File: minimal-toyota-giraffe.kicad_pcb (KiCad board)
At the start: 2 copper layers, 39.4 x 24.1 mm, 6 parts, among them J1 USB_A, J2 MOBILEEYE, J3 MOBILEEYE, P1 panda, U1 Power

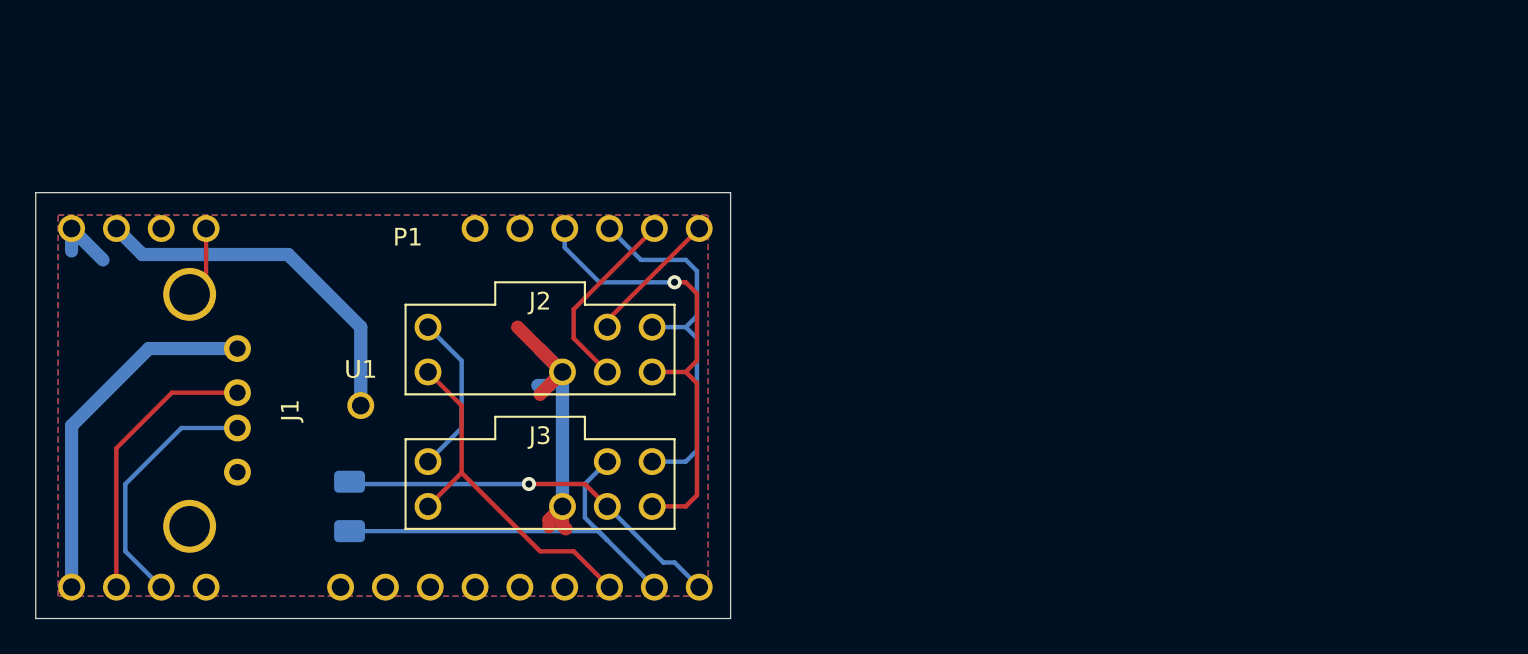
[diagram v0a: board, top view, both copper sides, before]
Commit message: new board design
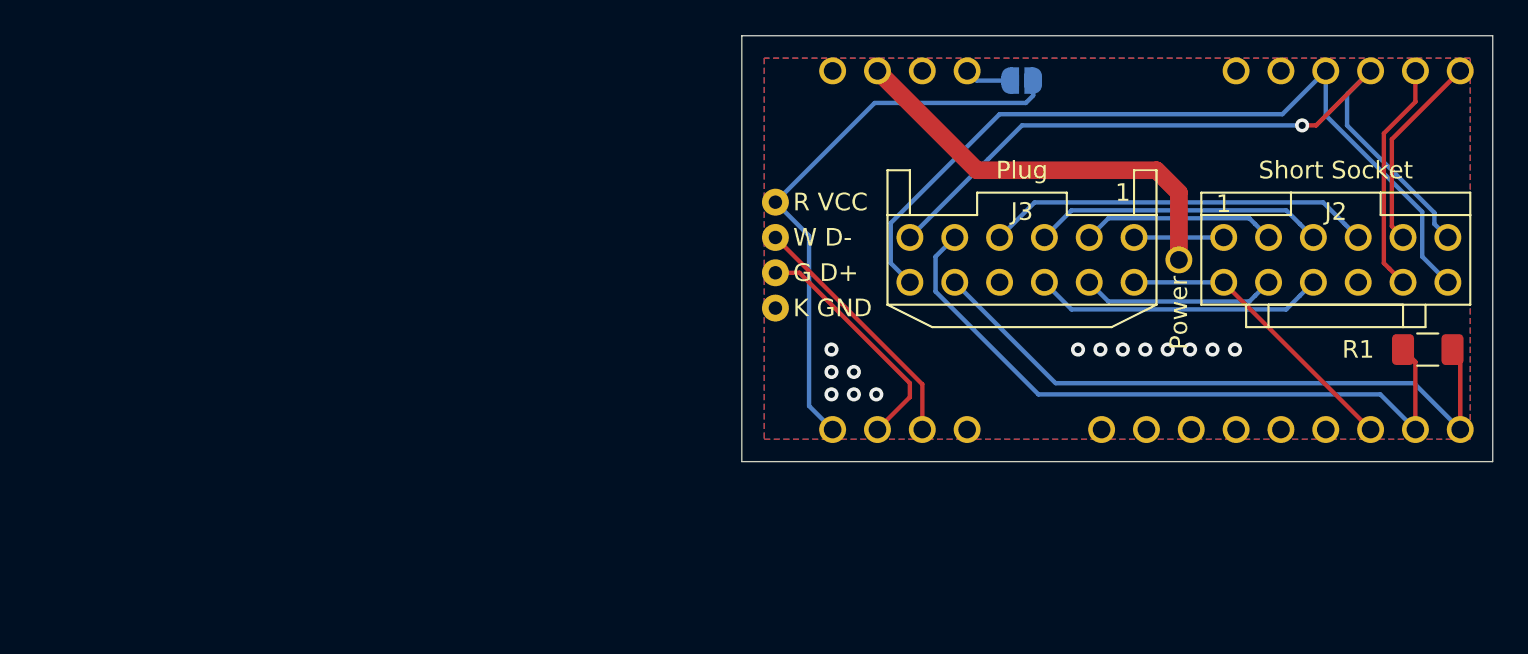
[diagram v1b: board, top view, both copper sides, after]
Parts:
- removed J1: USB_A, giraffe:USB
- added JP1: Paw_Boot, Jumper:SolderJumper-2_P1.3mm_Open_RoundedPad1.0x1.5mm, B.Cu at (116.8, 80.0)
- added U2: USB, giraffe:USB, F.Cu at (102.9, 89.9)
- R1: moved to F.Cu
- moved R1 61.7 mm to (139.8, 95.2), turned to 180 degrees
- moved U1 47.1 mm to (125.7, 90.2), turned to 270 degrees
- moved J2 45.4 mm to (134.6, 91.4)
- moved P1 44.0 mm to (106.1, 99.8)
- moved J3 26.9 mm to (111.8, 88.9), turned to 180 degrees
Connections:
- P1 pad 10: Net-(P1-Pad10) -> (no net)
- P1 pad 16: Net-(P1-Pad16) -> (no net)
- P1 pad 18: Net-(P1-Pad18) -> (no net)
- P1 pad 19: Net-(P1-Pad19) -> (no net)
- P1 pad 5: Net-(P1-Pad5) -> (no net)
- P1 pad 6: Net-(P1-Pad6) -> (no net)
- P1 pad 7: Net-(P1-Pad7) -> (no net)
- P1 pad 9: Net-(P1-Pad9) -> (no net)
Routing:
- net /GND: track 23.1 -> 0.00 mm, vias 0 -> 14
- net /4: track 0.00 -> 22.0 mm
- net /CAN2_H: track 21.3 -> 42.4 mm, vias 0 -> 1
- net /CAN2_L: track 26.3 -> 46.9 mm, vias 1 -> 0
- net /9: track 0.00 -> 16.5 mm
- net /3: track 0.00 -> 16.5 mm
- net /CAN1_H': track 24.1 -> 38.8 mm
- net /CAN1_L': track 22.3 -> 36.8 mm, vias 1 -> 0
- net Net-(JP1-Pad1): track 20.4 -> 32.2 mm
- net /8: track 0.00 -> 11.1 mm
- net /2: track 0.00 -> 11.1 mm
- net /HTR: track 9.20 -> 5.08 mm
- net /CAN1_H: track 7.74 -> 11.3 mm
- net /IGN: track 20.3 -> 16.9 mm
- net /12VIN: track 20.6 -> 23.7 mm
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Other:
- board size 39.4 x 24.1 mm -> 42.5 x 24.1 mm
